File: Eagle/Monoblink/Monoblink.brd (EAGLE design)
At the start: 16 x 30 mm, 6 parts, among them U1 ATTINY85

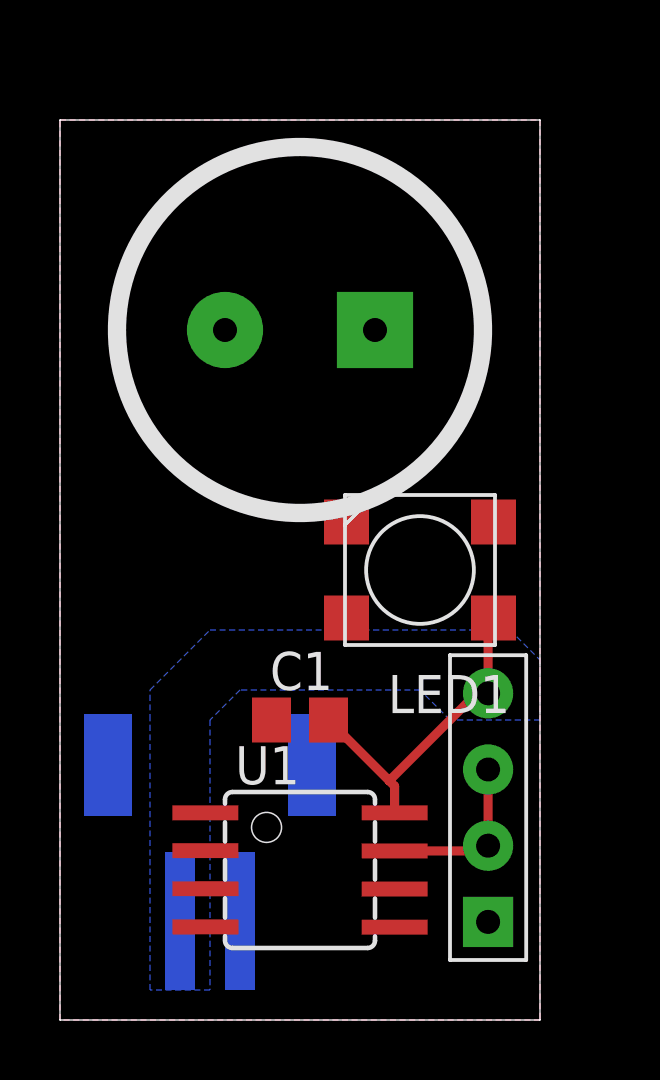
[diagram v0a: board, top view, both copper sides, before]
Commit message: rebleuble
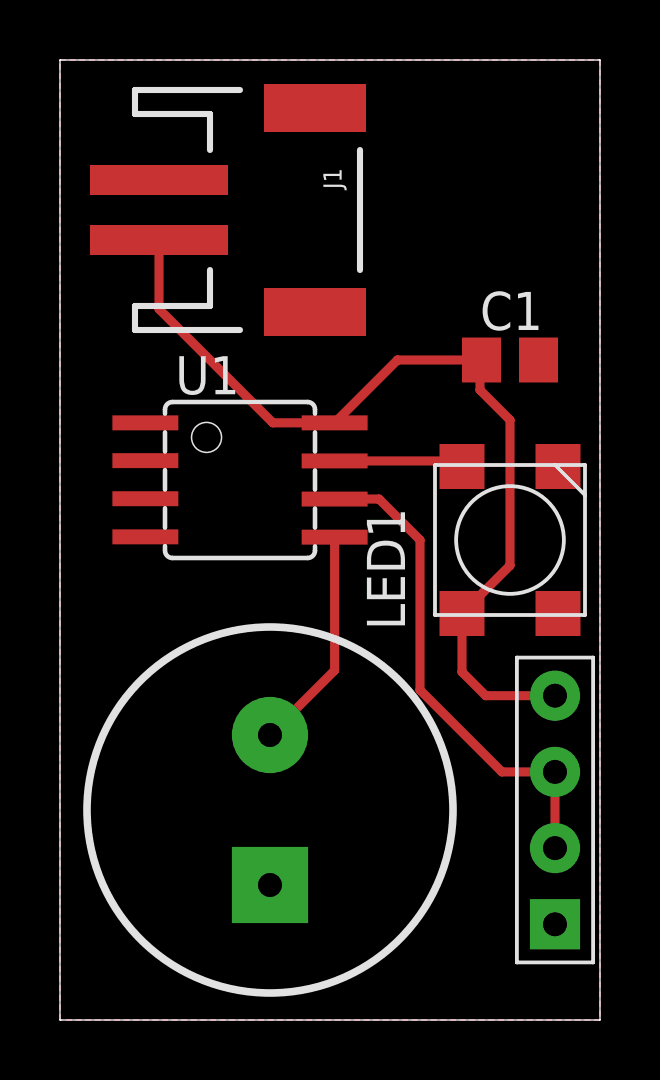
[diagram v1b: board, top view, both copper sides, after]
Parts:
- moved J1 20.1 mm to (7.00, 27.0), flipped to the top, turned to 270 degrees
- moved U$2 16.0 mm to (7.00, 7.00), turned to 0 degrees
- moved C1 13.9 mm to (15.0, 22.0), turned to 0 degrees
- moved U1 13.2 mm to (6.00, 18.0)
- moved U$1 6.10 mm to (16.5, 7.00)
- moved LED1 3.16 mm to (15.0, 16.0), turned to 90 degrees
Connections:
- net LED_DATA_IN: now also U1.7; no longer U1.6
- net RF_DATA_OUT: now also U1.6; no longer U1.7
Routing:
- net VCC: track 11.1 -> 30.4 mm
- net RF_DATA_OUT: track 5.73 -> 16.6 mm
- net PIEZO_IN: track 0.00 -> 7.49 mm
- net LED_DATA_IN: track 0.00 -> 4.32 mm
- removed copper zone on layer 16, net VCC
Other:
- board size 16 x 30 mm -> 18 x 32 mm
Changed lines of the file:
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@@
 <board>
 <plain>
-<wire x1="0" y1="0" x2="16" y2="0" width="0" layer="20"/>
-<wire x1="16" y1="0" x2="16" y2="30" width="0" layer="20"/>
-<wire x1="16" y1="30" x2="0" y2="30" width="0" layer="20"/>
-<wire x1="0" y1="30" x2="0" y2="0" width="0" layer="20"/>
+<wire x1="0" y1="0" x2="18" y2="0" width="0" layer="20"/>
+<wire x1="18" y1="0" x2="18" y2="32" width="0" layer="20"/>
+<wire x1="18" y1="32" x2="0" y2="32" width="0" layer="20"/>
+<wire x1="0" y1="32" x2="0" y2="0" width="0" layer="20"/>
 <polygon width="0.1524" layer="48" pour="hatch">
-<vertex x="16" y="30"/>
-<vertex x="30" y="30"/>
-<vertex x="30" y="0"/>
-<vertex x="16" y="0"/>
+<vertex x="18" y="32"/>
+<vertex x="32" y="32"/>
+<vertex x="32" y="0"/>
+<vertex x="18" y="0"/>
 </polygon>
-<rectangle x1="16" y1="2" x2="19" y2="12" layer="48"/>
+<rectangle x1="18" y1="2" x2="21" y2="12" layer="48"/>
 </plain>
 <attributes>
@@
 </autorouter>
 <elements>
-<element name="U1" library="Monoblink" package="SOIC8" value="ATTINY85" x="8" y="5" rot="R270"/>
-<element name="J1" library="Monoblink" package="JST-2-SMD" value="" x="5" y="7" rot="MR0">
-<attribute name="PROD_ID" value="CONN-11443" x="5" y="7" size="1.778" layer="28" rot="MR0" display="off"/>
-<attribute name="SF_ID" value="PRT-08612" x="5" y="7" size="1.778" layer="28" rot="MR0" display="off"/>
+<element name="U1" library="Monoblink" package="SOIC8" value="ATTINY85" x="6" y="18" rot="R270"/>
+<element name="J1" library="Monoblink" package="JST-2-SMD" value="" x="7" y="27" rot="R270">
+<attribute name="PROD_ID" value="CONN-11443" x="7" y="27" size="1.778" layer="27" rot="R270" display="off"/>
+<attribute name="SF_ID" value="PRT-08612" x="7" y="27" size="1.778" layer="27" rot="R270" display="off"/>
 </element>
-<element name="LED1" library="Monoblink" package="SMD5050" value="NEOPIXEL" x="12" y="15" rot="R180"/>
-<element name="U$1" library="Monoblink" package="RF_CONN" value="RF_CONN" x="13" y="2"/>
-<element name="C1" library="Monoblink" package="C0805" value="" x="8" y="10" smashed="yes" rot="R180">
-<attribute name="NAME" x="7" y="11" size="1.27" layer="25"/>
-<attribute name="SPICEPREFIX" value="C" x="8" y="10" size="1.778" layer="27" rot="R180" display="off"/>
-<attribute name="VALUE" x="9.27" y="12.54" size="1.27" layer="27" rot="R180"/>
+<element name="LED1" library="Monoblink" package="SMD5050" value="NEOPIXEL" x="15" y="16" rot="R90"/>
+<element name="U$1" library="Monoblink" package="RF_CONN" value="RF_CONN" x="16.5" y="7"/>
+<element name="C1" library="Monoblink" package="C0805" value="" x="15" y="22" smashed="yes">
+<attribute name="NAME" x="14" y="23" size="1.27" layer="25"/>
+<attribute name="SPICEPREFIX" value="C" x="15" y="22" size="1.778" layer="27" display="off"/>
+<attribute name="VALUE" x="13.73" y="19.46" size="1.27" layer="27"/>
 </element>
-<element name="U$2" library="Monoblink" package="PS1240P02BT" value="PIEZO" x="8" y="23" rot="R90"/>
+<element name="U$2" library="Monoblink" package="PS1240P02BT" value="PIEZO" x="7" y="7"/>
 </elements>
 <signals>
 <signal name="GND">
 <polygon width="0.1524" layer="1" rank="3">
-<vertex x="0" y="30"/>
-<vertex x="16" y="30"/>
-<vertex x="16" y="0"/>
+<vertex x="0" y="32"/>
+<vertex x="18" y="32"/>
+<vertex x="18" y="0"/>
 <vertex x="0" y="0"/>
 </polygon>
 <polygon width="0.1524" layer="16" rank="2">
-<vertex x="0" y="30"/>
-<vertex x="16" y="30"/>
-<vertex x="16" y="0"/>
+<vertex x="0" y="32"/>
+<vertex x="18" y="32"/>
+<vertex x="18" y="0"/>
 <vertex x="0" y="0"/>
 </polygon>
@@
 <contactref element="LED1" pad="3"/>
 <contactref element="C1" pad="1"/>
-<polygon width="0.1524" layer="16" thermals="no">
-<vertex x="13" y="10"/>
-<vertex x="12" y="11"/>
-<vertex x="6" y="11"/>
-<vertex x="5" y="10"/>
-<vertex x="5" y="1"/>
-<vertex x="3" y="1"/>
-<vertex x="3" y="10"/>
-<vertex x="3" y="11"/>
-<vertex x="5" y="13"/>
-<vertex x="15" y="13"/>
-<vertex x="16" y="12"/>
-<vertex x="16" y="10"/>
-</polygon>
-<wire x1="8.95" y1="10" x2="10.975" y2="7.975" width="0.3048" layer="1"/>
-<wire x1="10.975" y1="7.975" x2="11.154" y2="7.796" width="0.3048" layer="1"/>
-<wire x1="11.154" y1="7.796" x2="11.154" y2="6.905" width="0.3048" layer="1"/>
-<wire x1="10.975" y1="7.975" x2="13.89" y2="10.89" width="0.3048" layer="1"/>
-<wire x1="13.89" y1="10.89" x2="14.27" y2="10.89" width="0.3048" layer="1"/>
-<wire x1="14.27" y1="10.89" x2="14.27" y2="13.22" width="0.3048" layer="1"/>
-<wire x1="14.27" y1="13.22" x2="14.45" y2="13.4" width="0.3048" layer="1"/>
+<wire x1="13.4" y1="13.55" x2="13.4" y2="11.6" width="0.3048" layer="1"/>
+<wire x1="14.19" y1="10.81" x2="16.5" y2="10.81" width="0.3048" layer="1"/>
+<wire x1="13.4" y1="11.6" x2="14.19" y2="10.81" width="0.3048" layer="1"/>
+<wire x1="14.05" y1="22" x2="11.249" y2="22" width="0.3048" layer="1"/>
+<wire x1="11.249" y1="22" x2="9.154" y2="19.905" width="0.3048" layer="1"/>
+<wire x1="13.4" y1="13.55" x2="15" y2="15.15" width="0.3048" layer="1"/>
+<wire x1="15" y1="15.15" x2="15" y2="20" width="0.3048" layer="1"/>
+<wire x1="15" y1="20" x2="14" y2="21" width="0.3048" layer="1"/>
+<wire x1="14" y1="21" x2="14" y2="21.95" width="0.3048" layer="1"/>
+<wire x1="14" y1="21.95" x2="14.05" y2="22" width="0.3048" layer="1"/>
+<wire x1="3.3" y1="26" x2="3.3" y2="23.7" width="0.3048" layer="1"/>
+<wire x1="7.095" y1="19.905" x2="9.154" y2="19.905" width="0.3048" layer="1"/>
+<wire x1="3.3" y1="23.7" x2="7.095" y2="19.905" width="0.3048" layer="1"/>
 </signal>
 <signal name="RF_DATA_OUT">
 <contactref element="U$1" pad="2"/>
 <contactref element="U$1" pad="3"/>
-<contactref element="U1" pad="7"/>
-<wire x1="11.154" y1="5.635" x2="14.095" y2="5.635" width="0.3048" layer="1"/>
-<wire x1="14.095" y1="5.635" x2="14.27" y2="5.81" width="0.3048" layer="1"/>
-<wire x1="14.27" y1="8.35" x2="14.27" y2="5.81" width="0.3048" layer="1"/>
+<wire x1="16.5" y1="5.73" x2="16.5" y2="8.27" width="0.3048" layer="1"/>
+<contactref element="U1" pad="6"/>
+<wire x1="9.154" y1="17.365" x2="10.635" y2="17.365" width="0.3048" layer="1"/>
+<wire x1="10.635" y1="17.365" x2="12" y2="16" width="0.3048" layer="1"/>
+<wire x1="12" y1="16" x2="12" y2="11" width="0.3048" layer="1"/>
+<wire x1="12" y1="11" x2="14.73" y2="8.27" width="0.3048" layer="1"/>
+<wire x1="14.73" y1="8.27" x2="16.5" y2="8.27" width="0.3048" layer="1"/>
 </signal>
 <signal name="LED_DATA_IN">
 <contactref element="LED1" pad="2"/>
-<contactref element="U1" pad="6"/>
-<wire x1="11.154" y1="4.365" x2="9.55" y2="13.4" width="0" layer="19" extent="1-1"/>
+<contactref element="U1" pad="7"/>
+<wire x1="9.154" y1="18.635" x2="13.215" y2="18.635" width="0.3048" layer="1"/>
+<wire x1="13.215" y1="18.635" x2="13.4" y2="18.45" width="0.3048" layer="1"/>
 </signal>
 <signal name="LED_DATA_OUT">
@@
 <signal name="PIEZO_IN">
 <contactref element="U$2" pad="V+"/>
+<wire x1="9.154" y1="11.654" x2="7" y2="9.5" width="0.3048" layer="1"/>
 <contactref element="U1" pad="5"/>
-<wire x1="11.154" y1="3.095" x2="5.5" y2="23" width="0" layer="19" extent="1-1"/>
+<wire x1="9.154" y1="16.095" x2="9.154" y2="11.654" width="0.3048" layer="1"/>
 </signal>
 </signals>
